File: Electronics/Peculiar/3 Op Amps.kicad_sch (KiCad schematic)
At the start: 12 parts, among them U15 ${SIM.PARAMS}, U18 ${SIM.PARAMS}

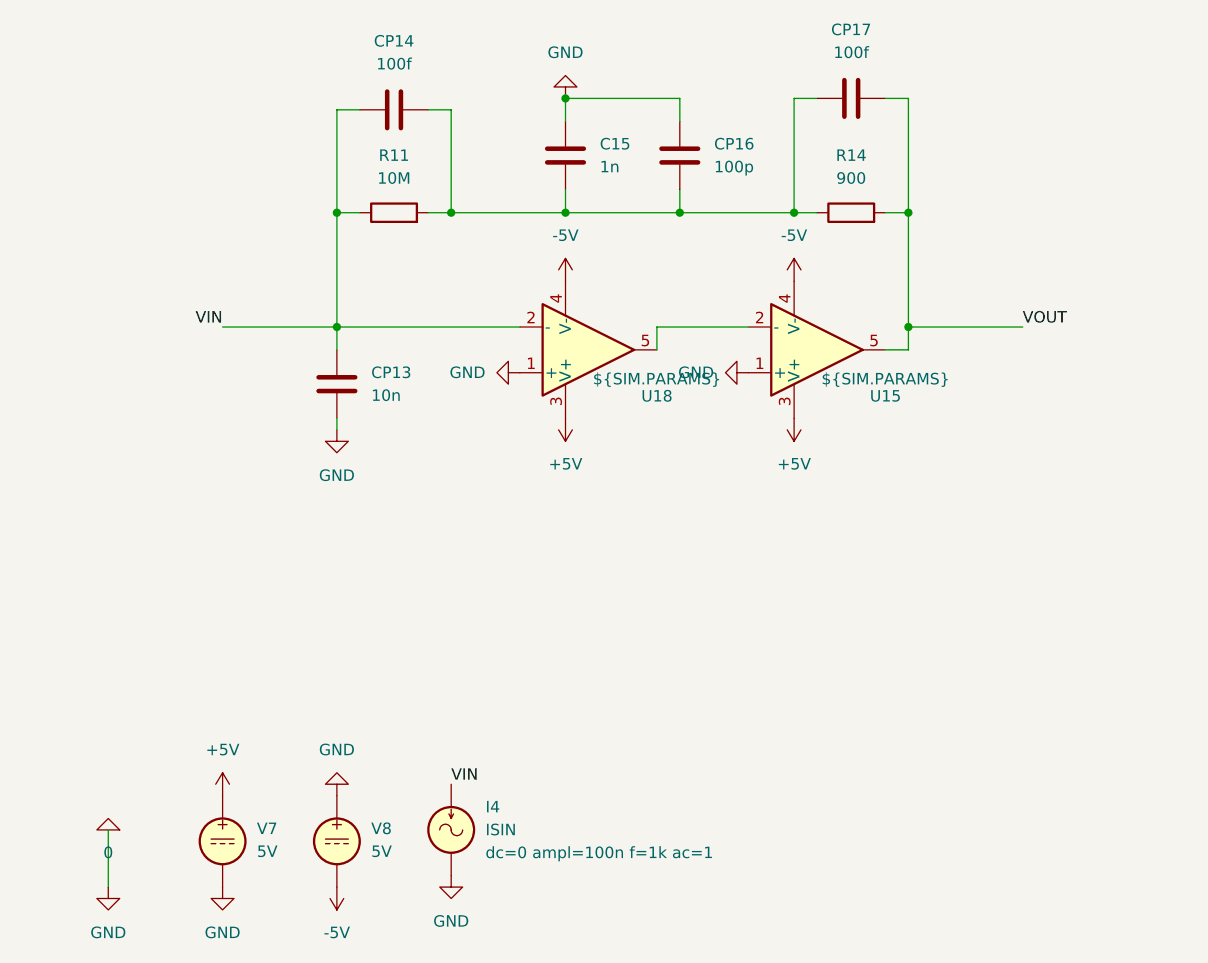
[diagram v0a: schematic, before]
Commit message: Create some other simulations
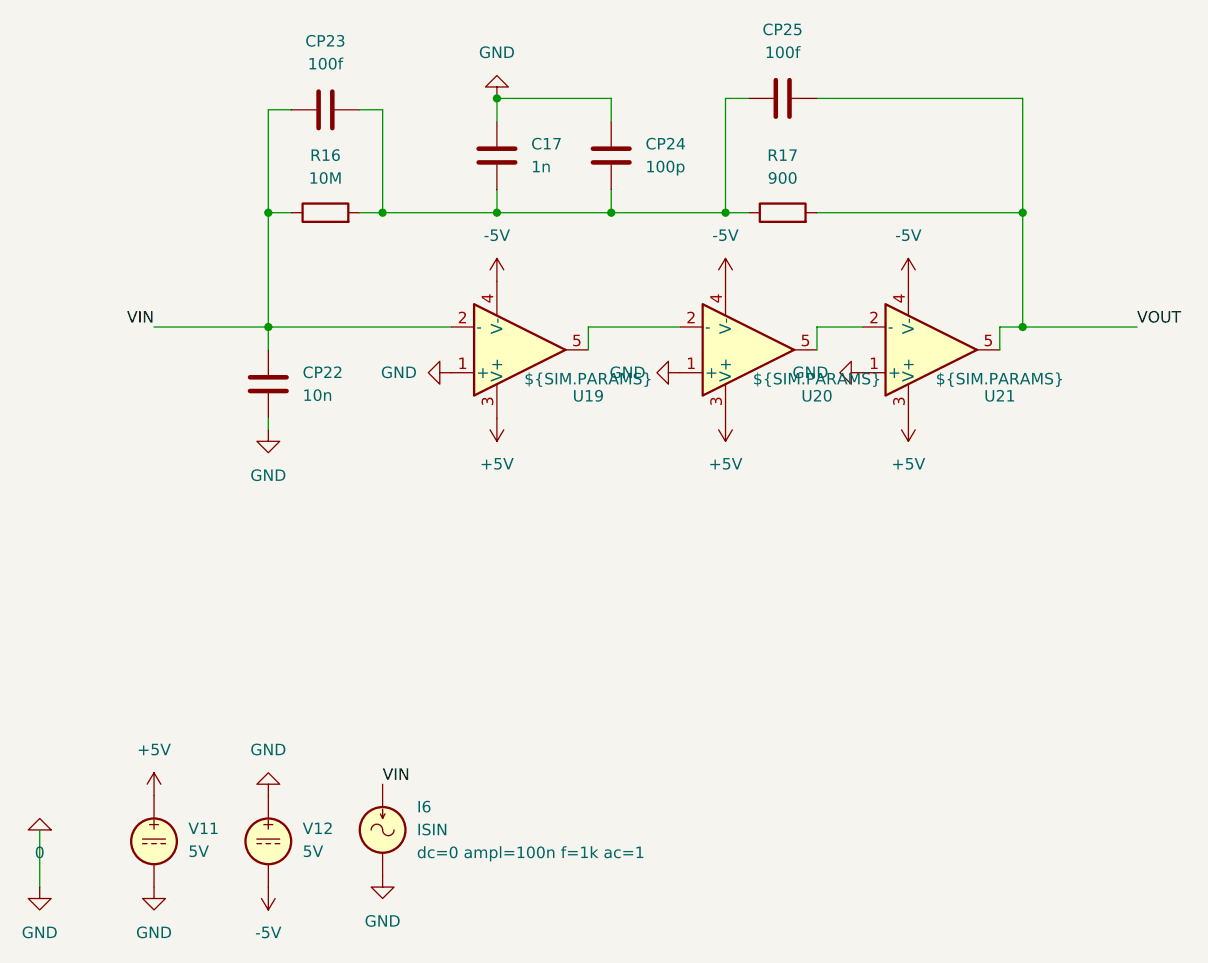
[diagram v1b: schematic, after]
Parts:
- removed C15: 1n, symbol Device:C
- removed CP13: 10n, symbol Device:C
- removed CP14, CP17: 100f, symbol Device:C
- removed CP16: 100p, symbol Device:C
- removed I4: ISIN, symbol Simulation_SPICE:ISIN
- removed R11: 10M, symbol Device:R
- removed R14: 900, symbol Device:R
- removed U15, U18: ${SIM.PARAMS}, symbol Simulation_SPICE:OPAMP
- removed V7, V8: 5V, symbol Simulation_SPICE:VDC
- added C17: 1n, symbol Device:C
- added CP22: 10n, symbol Device:C
- added CP23, CP25: 100f, symbol Device:C
- added CP24: 100p, symbol Device:C
- added I6: ISIN, symbol Simulation_SPICE:ISIN
- added R16: 10M, symbol Device:R
- added R17: 900, symbol Device:R
- added U19, U20, U21: ${SIM.PARAMS}, symbol Simulation_SPICE:OPAMP
- added V11, V12: 5V, symbol Simulation_SPICE:VDC
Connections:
- net +5V: now also U19.3 (V+), U20.3 (V+), U21.3 (V+), V11.1
- net -5V: now also U19.4 (V-), U20.4 (V-), U21.4 (V-), V12.2
- net 0: now also C17.2, CP22.2, CP24.2, I6.2, U19.1 (+), U20.1 (+), U21.1 (+), V11.2, V12.1
- net VIN: now also CP22.1, CP23.1, I6.1, R16.1, U19.2 (-)
- net VOUT: now also CP25.2, R17.2, U21.5
- new net: C17.1, CP23.2, CP24.1, CP25.1, R16.2, R17.1
- new net: U20.5, U21.2 (-)
- new net: U19.5, U20.2 (-)
